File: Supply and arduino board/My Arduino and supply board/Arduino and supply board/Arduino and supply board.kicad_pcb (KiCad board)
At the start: 2 copper layers, 49 x 64 mm, 70 parts, among them J1 USB_C_Receptacle_USB2.0, J2 Conn_01x03, J3 Conn_01x03, J4 Conn_01x03, J5 Conn_01x03, J6 Conn_01x03, J7 Conn_01x03, J8 Programing_port, J9 Conn_01x05, Q2 16MHz, U1 MP4581GN-P, U2 MP4581GN-P, U6 USBLC6-2P6, U7 Atmega328P-PU, U8 FT231XQ, Y2 16MHz

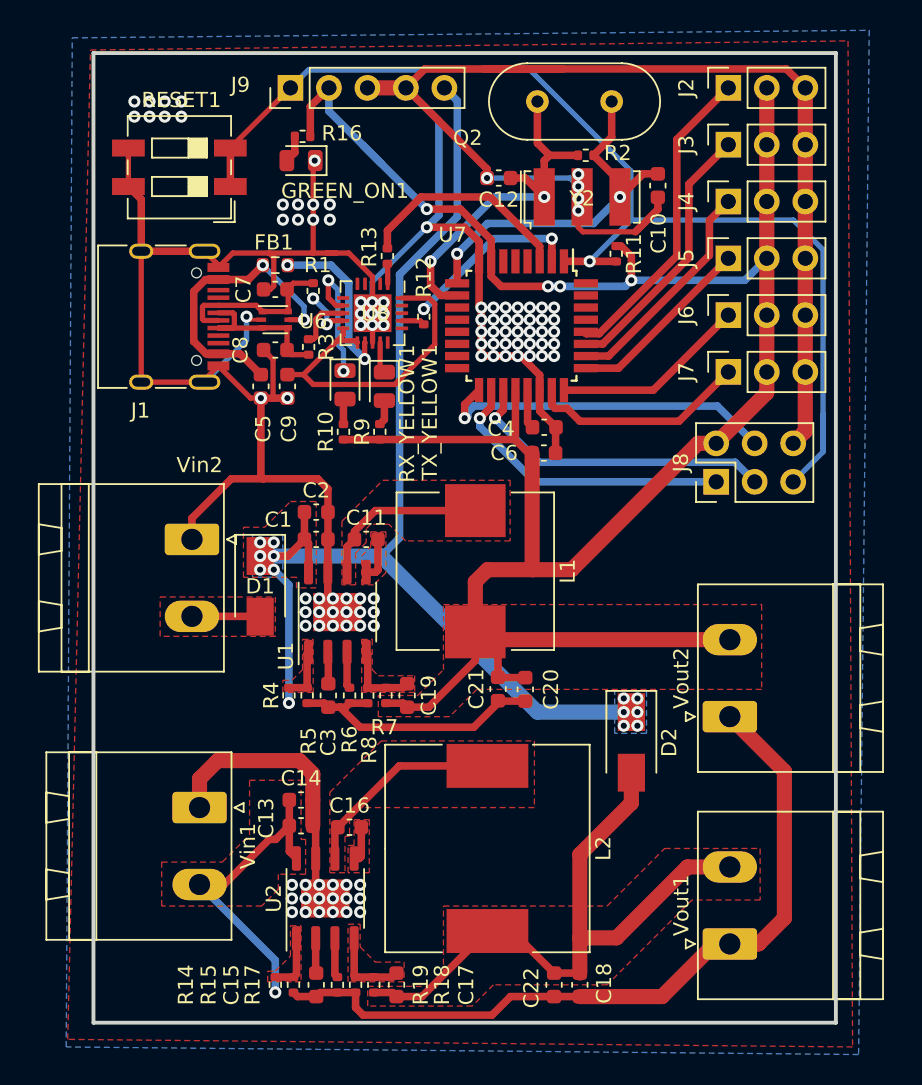
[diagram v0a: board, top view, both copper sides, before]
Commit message: changes on powersuply
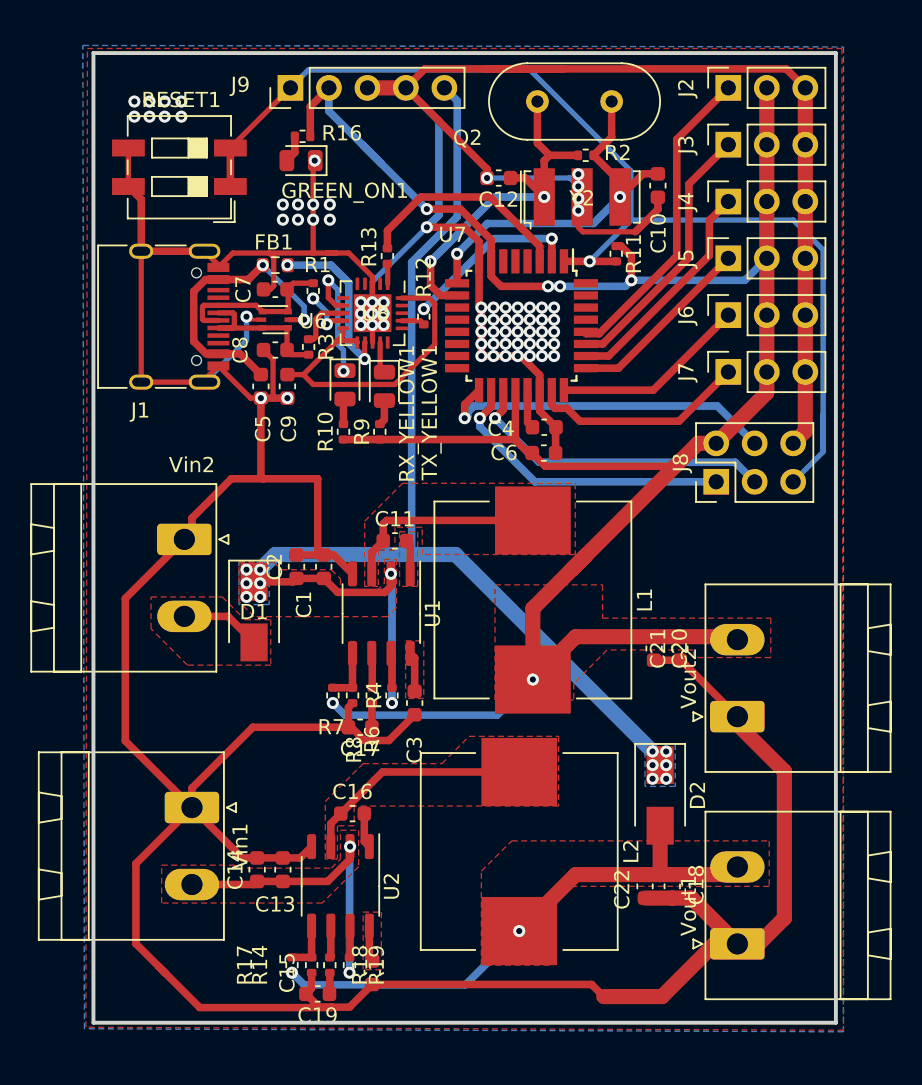
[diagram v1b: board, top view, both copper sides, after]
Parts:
- removed R15: 5.6K, Resistor_SMD:R_0402_1005Metric
- removed R5: 12K, Resistor_SMD:R_0402_1005Metric
- C15, C3: value 1u -> 0.1u
- C16: value 0.1u -> 10n
- C17: value 680p -> 3.9u
- C19: value 680p -> 3.9n
- L1: value 33u -> 220uH/1.6A; footprint Inductor_SMD:L_Wuerth_HCI-1040 -> Inductor_SMD:L_Wuerth_HCI-1350
- L2: value 47u -> 220uH/1.6A; footprint Inductor_SMD:L_Wuerth_HCM-1350 -> Inductor_SMD:L_Wuerth_HCI-1350
- R17: value 33K -> 6.8K
- R19: value 10K -> 9K
- R6: value 82K -> 6.8K
- R8: value 43K -> 2.4K
- U1, U2: value MP4581GN-P -> TD2786MR; footprint Package_SO:SOIC-8-1EP_3.9x4.9mm_P1.27mm_EP2.514x3.2mm -> Package_SO:SOP-8_3.9x4.9mm_P1.27mm
- moved C19 20.6 mm to (147.0, 106.1), turned to 180 degrees
- moved C17 17.2 mm to (149.8, 88.5), turned to 180 degrees
- moved C21 12.3 mm to (170.9, 83.3)
- moved C20 8.92 mm to (169.2, 83.3)
- moved C18 8.91 mm to (170.4, 99.0)
- moved C22 8.85 mm to (168.6, 99.0)
- moved R4 6.80 mm to (151.9, 86.4)
- moved C3 5.72 mm to (153.4, 86.9)
- moved R18 5.55 mm to (145.3, 104.2)
- moved C14 5.44 mm to (143.0, 97.9), turned to 90 degrees
- moved R14 5.07 mm to (149.1, 104.2)
- moved L1 4.25 mm to (161.2, 80.1)
- moved D2 3.98 mm to (169.6, 93.0)
- moved C2 3.83 mm to (145.6, 77.9), turned to 90 degrees
- moved C15 3.79 mm to (150.6, 104.7)
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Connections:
- C17 pad 2: /VOUT+12V -> GND
- C19 pad 2: +5V -> GND
- R17 pad 2: GND -> Net-(C19-Pad1)
- R18 pad 2: Net-(C17-Pad1) -> Net-(R18-Pad2)
- R19 pad 1: Net-(C17-Pad1) -> Net-(R18-Pad2)
- R6 pad 2: GND -> Net-(C17-Pad1)
- R7 pad 2: Net-(C19-Pad1) -> Net-(R7-Pad2)
- R8 pad 1: Net-(C19-Pad1) -> Net-(R7-Pad2)
- U1 pad 1: Net-(R4-Pad2) -> Net-(C11-Pad2)
- U1 pad 2: Net-(C3-Pad1) -> /VIN+12V
- U1 pad 3: Net-(R6-Pad1) -> Net-(C11-Pad1)
- U1 pad 4: Net-(C19-Pad1) -> GND
- U1 pad 5: Net-(C11-Pad2) -> Net-(R7-Pad2)
- U1 pad 6: Net-(C11-Pad1) -> Net-(R6-Pad1)
- U1 pad 7: GND -> Net-(R4-Pad2)
- U1 pad 8: /VIN+12V -> Net-(C3-Pad1)
- U2 pad 1: Net-(R14-Pad2) -> Net-(C16-Pad2)
- U2 pad 2: Net-(C15-Pad1) -> /VIN+24V
- U2 pad 3: Net-(R17-Pad1) -> Net-(C16-Pad1)
- U2 pad 4: Net-(C17-Pad1) -> GND
- U2 pad 5: Net-(C16-Pad2) -> Net-(R18-Pad2)
- U2 pad 6: Net-(C16-Pad1) -> Net-(R17-Pad1)
- U2 pad 7: GND -> Net-(R14-Pad2)
- U2 pad 8: /VIN+24V -> Net-(C15-Pad1)
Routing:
- net GND: track 300.9 -> 355.8 mm, vias 106 -> 70
- net /VOUT+12V: track 43.1 -> 36.2 mm, vias 0 -> 2
- net Net-(C17-Pad1): track 5.40 -> 1.60 mm
- net Net-(C19-Pad1): track 5.12 -> 1.40 mm
- net Net-(R7-Pad2): track 0.00 -> 3.57 mm
- net Net-(R18-Pad2): track 0.00 -> 3.37 mm
- net Net-(C11-Pad1): track 11.4 -> 13.6 mm
- net Net-(R14-Pad2): track 3.83 -> 2.08 mm
- net Net-(C16-Pad1): track 13.7 -> 15.4 mm
- net Net-(R4-Pad2): track 3.59 -> 2.29 mm
- net Net-(D1-Pad2): track 4.51 -> 5.31 mm
- net /VIN+12V: track 82.5 -> 83.2 mm, vias 13 -> 14
- net Net-(C11-Pad2): track 2.85 -> 2.27 mm
- net +5V: track 149.1 -> 148.5 mm, vias 4 -> 6
- net Net-(R17-Pad1): track 2.62 -> 2.09 mm
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- added copper zone on F.Cu, net Net-(C15-Pad1)
- added copper zone on F.Cu, net Net-(C3-Pad1)
- removed copper zone on F.Cu, net Net-(C16-Pad2)
- removed copper zone on F.Cu, net Net-(C17-Pad1)
- removed copper zone on F.Cu, net Net-(C19-Pad1)
- removed copper zone on F.Cu, net Net-(R14-Pad2)
- removed copper zone on F.Cu, net Net-(R4-Pad2)
